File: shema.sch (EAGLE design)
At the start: 20 parts

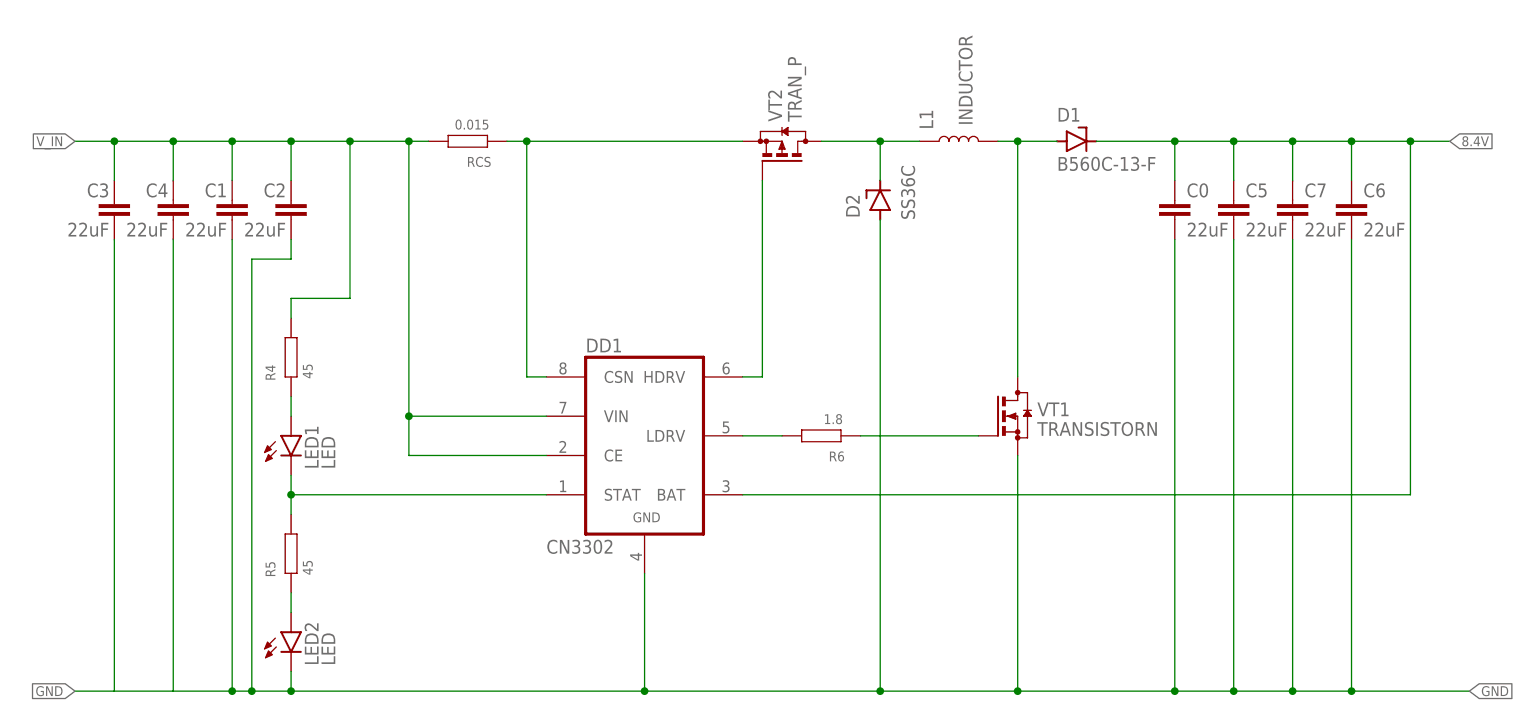
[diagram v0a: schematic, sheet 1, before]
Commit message: изменения файлов
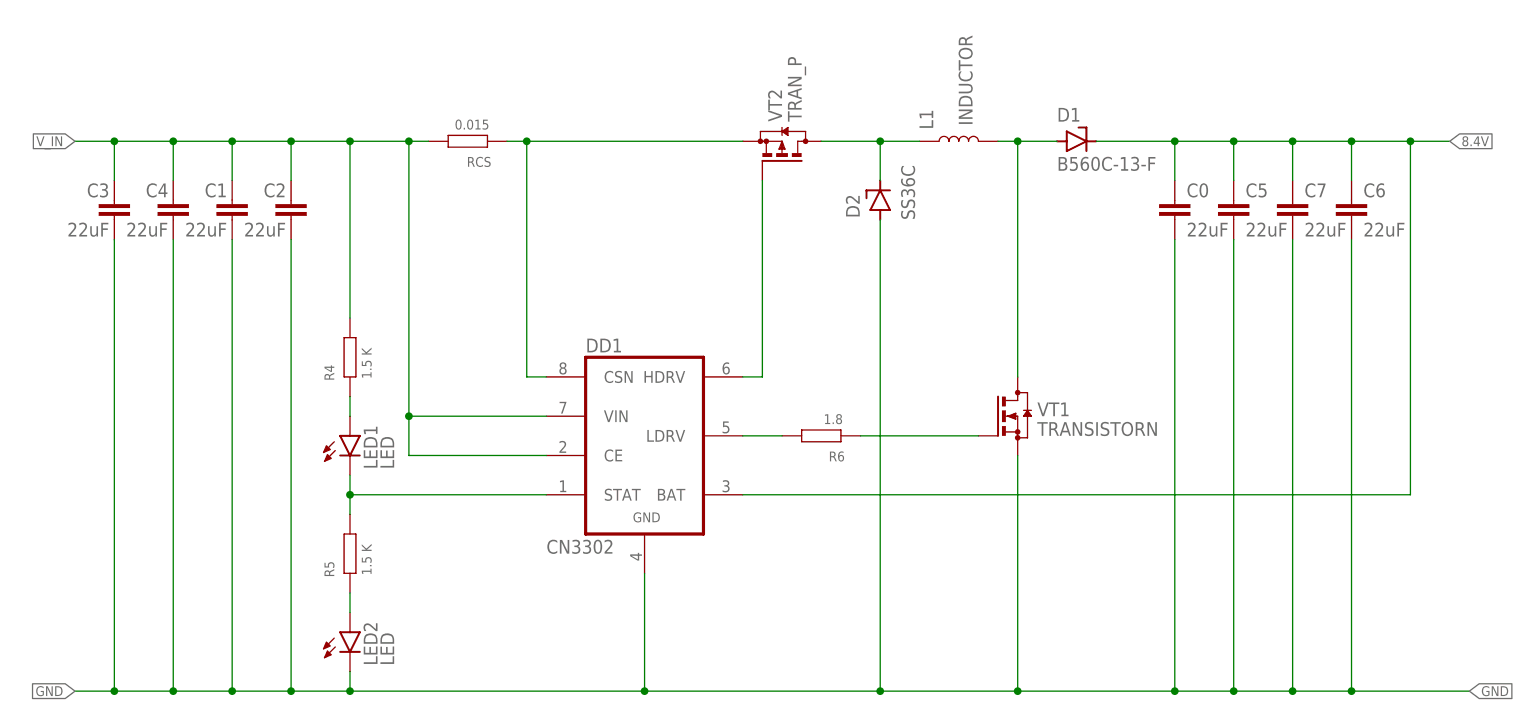
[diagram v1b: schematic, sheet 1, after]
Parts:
- R4, R5: value 45 -> 1.5 K
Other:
- moved on the sheet: LED1, LED2, R4, R5
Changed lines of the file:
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@@
 <attribute name="SPICEPREFIX" value="C"/>
 </part>
-<part name="R4" library="1_RESISTOR" deviceset="RESISTOR" device="0603" value="45"/>
-<part name="R5" library="1_RESISTOR" deviceset="RESISTOR" device="0603" value="45"/>
+<part name="R4" library="1_RESISTOR" deviceset="RESISTOR" device="0603" value="1.5 K"/>
+<part name="R5" library="1_RESISTOR" deviceset="RESISTOR" device="0603" value="1.5 K"/>
 <part name="R6" library="1_RESISTOR" deviceset="RESISTOR" device="0603" value="1.8"/>
 </parts>
@@
 <attribute name="VALUE" x="50.8" y="2.54" size="1.778" layer="96"/>
 </instance>
-<instance part="LED1" gate="G$1" x="-45.72" y="2.54" smashed="yes">
-<attribute name="NAME" x="-42.164" y="-1.778" size="1.778" layer="95" rot="R90"/>
-<attribute name="VALUE" x="-40.005" y="-1.778" size="1.778" layer="96" rot="R90"/>
-</instance>
-<instance part="LED2" gate="G$1" x="-45.72" y="-22.86" smashed="yes">
-<attribute name="NAME" x="-42.164" y="-27.178" size="1.778" layer="95" rot="R90"/>
-<attribute name="VALUE" x="-40.005" y="-27.178" size="1.778" layer="96" rot="R90"/>
+<instance part="LED1" gate="G$1" x="-38.1" y="2.54" smashed="yes">
+<attribute name="NAME" x="-34.544" y="-1.778" size="1.778" layer="95" rot="R90"/>
+<attribute name="VALUE" x="-32.385" y="-1.778" size="1.778" layer="96" rot="R90"/>
+</instance>
+<instance part="LED2" gate="G$1" x="-38.1" y="-22.86" smashed="yes">
+<attribute name="NAME" x="-34.544" y="-27.178" size="1.778" layer="95" rot="R90"/>
+<attribute name="VALUE" x="-32.385" y="-27.178" size="1.778" layer="96" rot="R90"/>
 </instance>
 <instance part="RCS" gate="G$1" x="-22.86" y="40.64" smashed="yes" rot="R180">
@@
 <attribute name="VALUE" x="85.344" y="28.321" size="1.778" layer="96"/>
 </instance>
-<instance part="R4" gate="G$1" x="-45.72" y="12.7" smashed="yes" rot="R90">
-<attribute name="VALUE" x="-42.926" y="9.906" size="1.27" layer="96" rot="R90"/>
-<attribute name="NAME" x="-47.752" y="9.652" size="1.27" layer="95" rot="R90"/>
-</instance>
-<instance part="R5" gate="G$1" x="-45.72" y="-12.7" smashed="yes" rot="R90">
-<attribute name="VALUE" x="-42.926" y="-15.494" size="1.27" layer="96" rot="R90"/>
-<attribute name="NAME" x="-47.752" y="-15.748" size="1.27" layer="95" rot="R90"/>
+<instance part="R4" gate="G$1" x="-38.1" y="12.7" smashed="yes" rot="R90">
+<attribute name="VALUE" x="-35.306" y="9.906" size="1.27" layer="96" rot="R90"/>
+<attribute name="NAME" x="-40.132" y="9.652" size="1.27" layer="95" rot="R90"/>
+</instance>
+<instance part="R5" gate="G$1" x="-38.1" y="-12.7" smashed="yes" rot="R90">
+<attribute name="VALUE" x="-35.306" y="-15.494" size="1.27" layer="96" rot="R90"/>
+<attribute name="NAME" x="-40.132" y="-15.748" size="1.27" layer="95" rot="R90"/>
 </instance>
 <instance part="R6" gate="G$1" x="22.86" y="2.54" smashed="yes" rot="R180">
@@
 <junction x="-45.72" y="40.64"/>
 <pinref part="R4" gate="G$1" pin="P$2"/>
-<wire x1="-45.72" y1="17.78" x2="-45.72" y2="20.32" width="0.1524" layer="91"/>
-<wire x1="-45.72" y1="20.32" x2="-38.1" y2="20.32" width="0.1524" layer="91"/>
-<wire x1="-38.1" y1="20.32" x2="-38.1" y2="40.64" width="0.1524" layer="91"/>
+<wire x1="-38.1" y1="17.78" x2="-38.1" y2="40.64" width="0.1524" layer="91"/>
 <junction x="-38.1" y="40.64"/>
 </segment>
@@
 <junction x="30.48" y="-30.48"/>
 <wire x1="0" y1="-15.24" x2="0" y2="-30.48" width="0.1524" layer="91"/>
-<wire x1="0" y1="-30.48" x2="-45.72" y2="-30.48" width="0.1524" layer="91"/>
+<wire x1="0" y1="-30.48" x2="-38.1" y2="-30.48" width="0.1524" layer="91"/>
 <junction x="0" y="-30.48"/>
-<wire x1="-45.72" y1="-30.48" x2="-50.8" y2="-30.48" width="0.1524" layer="91"/>
-<wire x1="-50.8" y1="-30.48" x2="-53.34" y2="-30.48" width="0.1524" layer="91"/>
+<wire x1="-38.1" y1="-30.48" x2="-45.72" y2="-30.48" width="0.1524" layer="91"/>
+<wire x1="-45.72" y1="-30.48" x2="-53.34" y2="-30.48" width="0.1524" layer="91"/>
 <wire x1="-53.34" y1="-30.48" x2="-60.96" y2="-30.48" width="0.1524" layer="91"/>
+<pinref part="LED2" gate="G$1" pin="C"/>
 <wire x1="-60.96" y1="-30.48" x2="-68.58" y2="-30.48" width="0.1524" layer="91"/>
 <wire x1="-68.58" y1="-30.48" x2="-73.66" y2="-30.48" width="0.1524" layer="91"/>
-<pinref part="LED2" gate="G$1" pin="C"/>
-<wire x1="-45.72" y1="-27.94" x2="-45.72" y2="-30.48" width="0.1524" layer="91"/>
-<junction x="-45.72" y="-30.48"/>
-<pinref part="C4" gate="G$1" pin="2"/>
-<wire x1="-60.96" y1="27.94" x2="-60.96" y2="-30.48" width="0.1524" layer="91"/>
-<pinref part="C3" gate="G$1" pin="2"/>
-<wire x1="-68.58" y1="27.94" x2="-68.58" y2="-30.48" width="0.1524" layer="91"/>
+<wire x1="-38.1" y1="-27.94" x2="-38.1" y2="-30.48" width="0.1524" layer="91"/>
+<junction x="-38.1" y="-30.48"/>
 <pinref part="C0" gate="G$1" pin="2"/>
 <wire x1="68.58" y1="27.94" x2="68.58" y2="-30.48" width="0.1524" layer="91"/>
@@
 <junction x="91.44" y="-30.48"/>
 <pinref part="C2" gate="G$1" pin="2"/>
-<wire x1="-45.72" y1="27.94" x2="-45.72" y2="25.4" width="0.1524" layer="91"/>
-<wire x1="-45.72" y1="25.4" x2="-50.8" y2="25.4" width="0.1524" layer="91"/>
-<wire x1="-50.8" y1="25.4" x2="-50.8" y2="-30.48" width="0.1524" layer="91"/>
-<junction x="-50.8" y="-30.48"/>
+<wire x1="-45.72" y1="27.94" x2="-45.72" y2="-30.48" width="0.1524" layer="91"/>
+<junction x="-45.72" y="-30.48"/>
 <pinref part="C1" gate="G$1" pin="2"/>
 <wire x1="-53.34" y1="27.94" x2="-53.34" y2="-30.48" width="0.1524" layer="91"/>
 <junction x="-53.34" y="-30.48"/>
+<pinref part="C3" gate="G$1" pin="2"/>
+<wire x1="-68.58" y1="27.94" x2="-68.58" y2="-30.48" width="0.1524" layer="91"/>
+<junction x="-68.58" y="-30.48"/>
+<pinref part="C4" gate="G$1" pin="2"/>
+<wire x1="-60.96" y1="27.94" x2="-60.96" y2="-30.48" width="0.1524" layer="91"/>
+<junction x="-60.96" y="-30.48"/>
 </segment>
 </net>
@@
 <segment>
 <pinref part="LED2" gate="G$1" pin="A"/>
-<wire x1="-45.72" y1="-20.32" x2="-45.72" y2="-17.78" width="0.1524" layer="91"/>
 <pinref part="R5" gate="G$1" pin="P$1"/>
+<wire x1="-38.1" y1="-17.78" x2="-38.1" y2="-20.32" width="0.1524" layer="91"/>
 </segment>
 </net>
@@
 <segment>
 <pinref part="LED1" gate="G$1" pin="C"/>
-<wire x1="-45.72" y1="-7.62" x2="-45.72" y2="-5.08" width="0.1524" layer="91"/>
+<wire x1="-38.1" y1="-7.62" x2="-38.1" y2="-5.08" width="0.1524" layer="91"/>
+<pinref part="R5" gate="G$1" pin="P$2"/>
 <pinref part="DD1" gate="CN" pin="STAT"/>
-<wire x1="-45.72" y1="-5.08" x2="-45.72" y2="-2.54" width="0.1524" layer="91"/>
-<wire x1="-12.7" y1="-5.08" x2="-45.72" y2="-5.08" width="0.1524" layer="91"/>
-<junction x="-45.72" y="-5.08"/>
-<pinref part="R5" gate="G$1" pin="P$2"/>
+<wire x1="-38.1" y1="-5.08" x2="-38.1" y2="-2.54" width="0.1524" layer="91"/>
+<wire x1="-12.7" y1="-5.08" x2="-38.1" y2="-5.08" width="0.1524" layer="91"/>
+<junction x="-38.1" y="-5.08"/>
 </segment>
 </net>
@@
 <segment>
 <pinref part="LED1" gate="G$1" pin="A"/>
-<wire x1="-45.72" y1="5.08" x2="-45.72" y2="7.62" width="0.1524" layer="91"/>
+<wire x1="-38.1" y1="5.08" x2="-38.1" y2="7.62" width="0.1524" layer="91"/>
 <pinref part="R4" gate="G$1" pin="P$1"/>
 </segment>
